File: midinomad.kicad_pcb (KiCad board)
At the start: 2 copper layers, 169.1 x 87.3 mm, 59 parts, among them J1 MIDI IN, J2 MIDI OUT, J3 Nomad 5pin, J4 Nomad 100, J7 DC IN, U1 6N138, U2 L7805, U3 74HC4053, U4 74HC4053

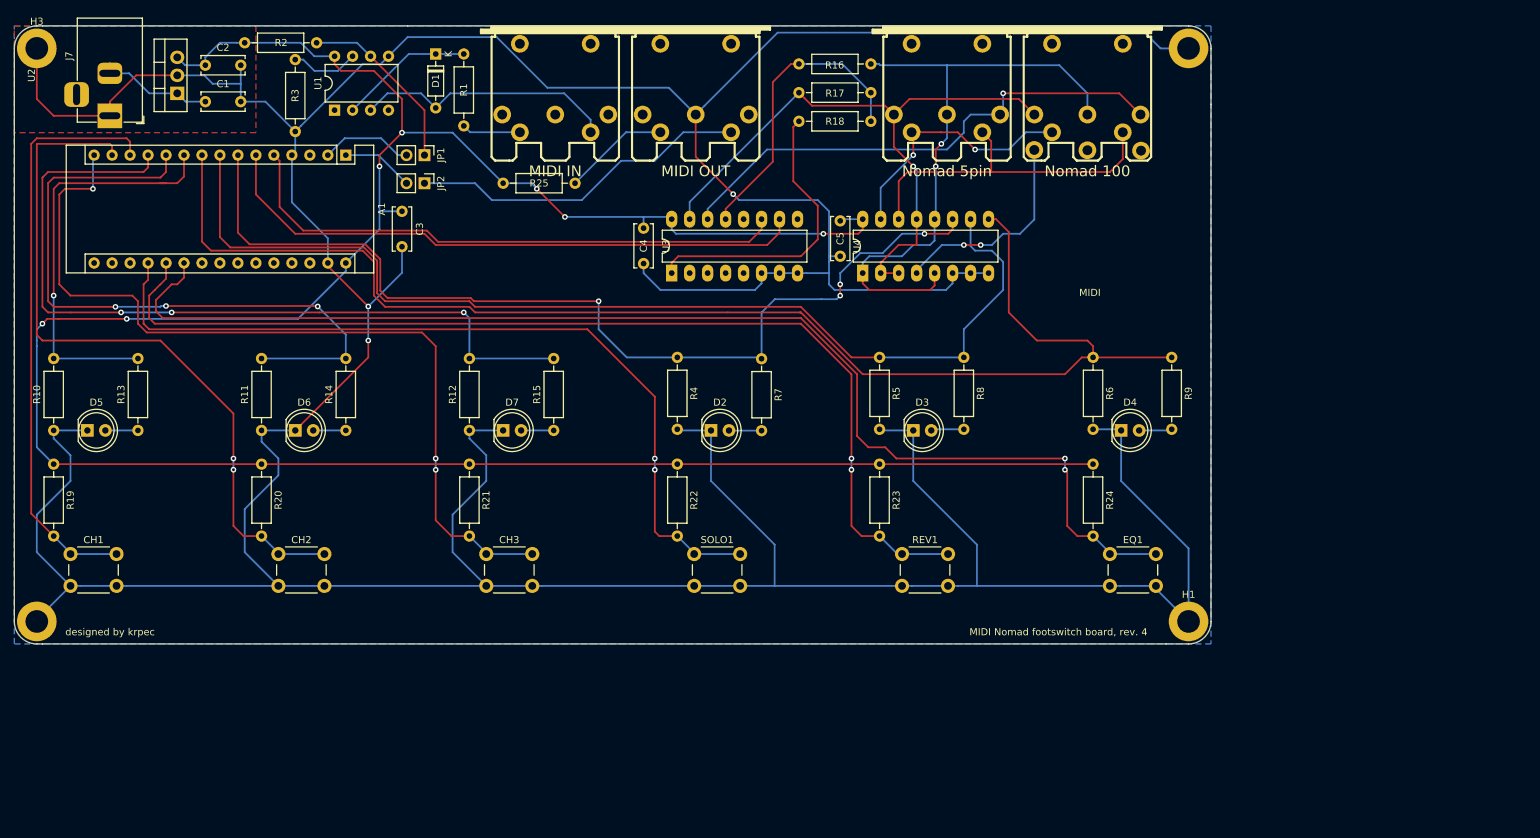
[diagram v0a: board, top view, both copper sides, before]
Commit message: Rev. 6 PCB & schematics
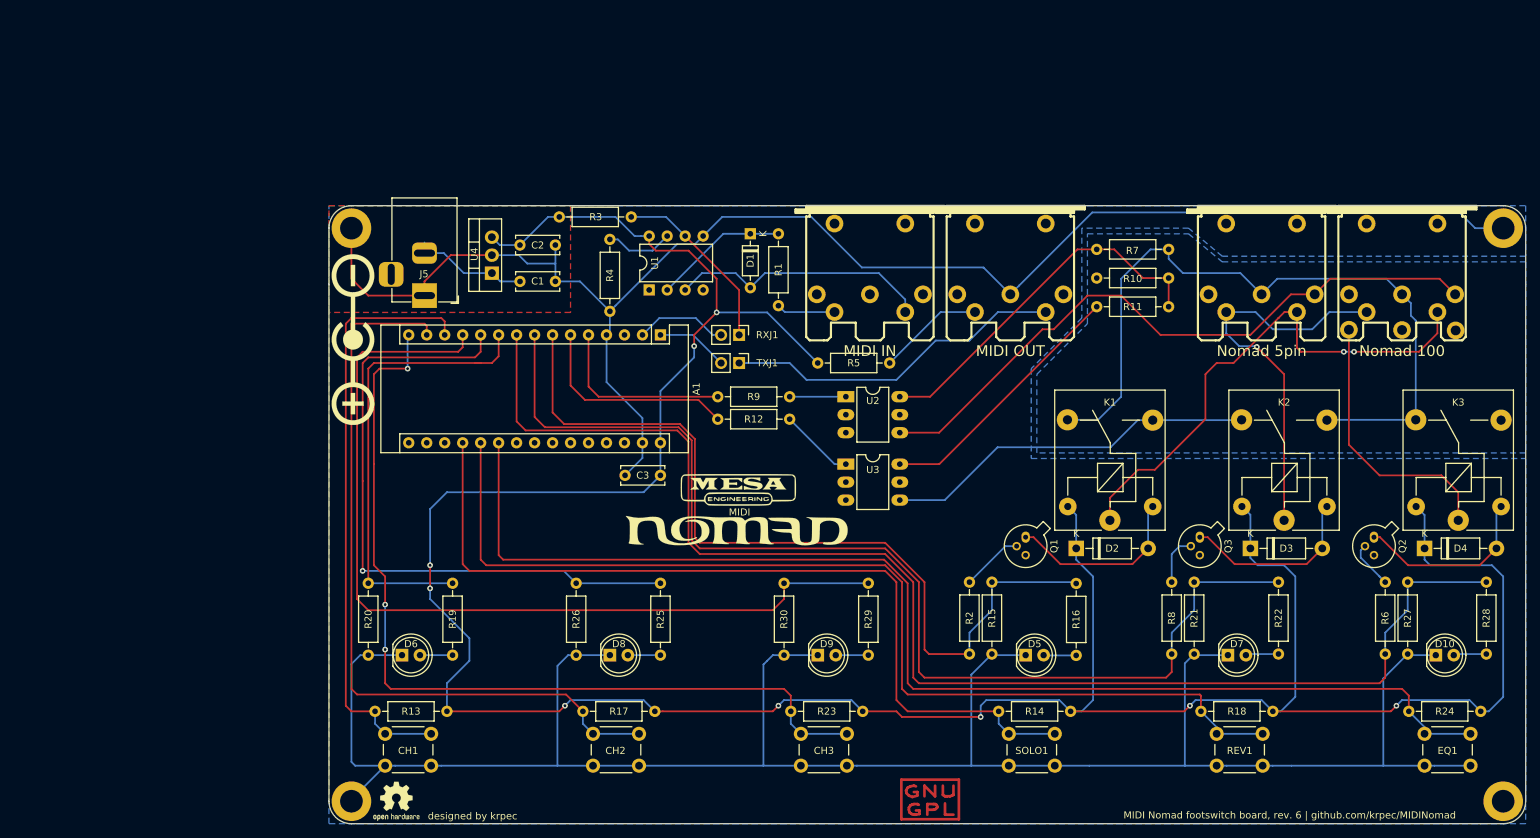
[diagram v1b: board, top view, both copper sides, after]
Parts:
- removed C4, C5: 0.1uF, Capacitor_THT:C_Disc_D6.0mm_W2.5mm_P5.00mm
- removed the U4 at (139.7, 57.1)
- added D10: LED, LED_THT:LED_D5.0mm, F.Cu at (220.7, 111.1)
- added D2: 1N4007, Diode_THT:D_DO-41_SOD81_P10.16mm_Horizontal, F.Cu at (169.9, 96.0)
- added D3: 1N4007, Diode_THT:D_DO-41_SOD81_P10.16mm_Horizontal, F.Cu at (194.5, 96.0)
- added G***: LOGO, midinomad-mux:board-logo, F.Cu at (122.2, 89.7)
- added K1: SANYOU_SRD_Form_C, Relay_THT:Relay_SPDT_SANYOU_SRD_Series_Form_C, F.Cu at (174.6, 92.1)
- added K2: SANYOU_SRD_Form_C, Relay_THT:Relay_SPDT_SANYOU_SRD_Series_Form_C, F.Cu at (199.2, 92.1)
- added K3: SANYOU_SRD_Form_C, Relay_THT:Relay_SPDT_SANYOU_SRD_Series_Form_C, F.Cu at (223.8, 92.1)
- added Q1: 2N2222, Package_TO_SOT_THT:TO-18-3, F.Cu at (162.7, 94.5)
- added Q2: 2N2222, Package_TO_SOT_THT:TO-18-3, F.Cu at (211.9, 94.5)
- added Q3: 2N2222, Package_TO_SOT_THT:TO-18-3, F.Cu at (187.3, 94.5)
- added R12: 220R, Resistor_THT:R_Axial_DIN0207_L6.3mm_D2.5mm_P10.16mm_Horizontal, F.Cu at (129.4, 77.8)
- added R2: 1k, Resistor_THT:R_Axial_DIN0207_L6.3mm_D2.5mm_P10.16mm_Horizontal, F.Cu at (154.8, 100.8)
- added R27: 10k, Resistor_THT:R_Axial_DIN0207_L6.3mm_D2.5mm_P10.16mm_Horizontal, F.Cu at (216.7, 100.8)
- added R28: 220R, Resistor_THT:R_Axial_DIN0207_L6.3mm_D2.5mm_P10.16mm_Horizontal, F.Cu at (227.8, 100.8)
- added R8: 1k, Resistor_THT:R_Axial_DIN0207_L6.3mm_D2.5mm_P10.16mm_Horizontal, F.Cu at (183.4, 100.8)
- added REF**: Symbol_GNU-GPL_CopperTop_Small, Symbol:Symbol_GNU-GPL_CopperTop_Small, F.Cu at (149.2, 131.8)
- added REF**: Polarity_Center_Negative_6mm_SilkScreen, Symbol:Polarity_Center_Negative_6mm_SilkScreen, F.Cu at (67.7, 66.5)
- added REF**: OSHW-Logo2_7.3x6mm_SilkScreen, Symbol:OSHW-Logo2_7.3x6mm_SilkScreen, F.Cu at (73.8, 131.8)
- added U2: MOC3041M, Package_DIP:DIP-6_W7.62mm_LongPads, F.Cu at (137.3, 74.6)
- D4: value LED -> 1N4007; footprint LED_THT:LED_D5.0mm -> Diode_THT:D_DO-41_SOD81_P10.16mm_Horizontal
- R6: value 10k -> 1k
- U3: value 74HC4053 -> MOC3041M; footprint Package_DIP:DIP-16_W7.62mm_LongPads -> Package_DIP:DIP-6_W7.62mm_LongPads
- moved R13 65.6 mm to (81.0, 119.1), turned to 180 degrees
- moved R14 65.6 mm to (169.1, 119.1), turned to 180 degrees
- moved R17 65.6 mm to (110.3, 119.1), turned to 180 degrees
- moved R18 65.6 mm to (197.6, 119.1), turned to 180 degrees
- moved R23 65.6 mm to (139.7, 119.1), turned to 180 degrees
- moved R24 65.0 mm to (227.0, 119.1), turned to 180 degrees
- moved R15 54.6 mm to (158.0, 100.8)
- moved R16 54.6 mm to (169.9, 101.0)
- moved D5 54.6 mm to (162.7, 111.1)
- moved D8 54.6 mm to (104.0, 111.1)
- moved R25 54.6 mm to (111.1, 111.1)
- moved R26 54.6 mm to (99.2, 111.1)
- moved R29 54.6 mm to (140.5, 111.1)
- moved R30 54.6 mm to (128.6, 111.1)
- moved D6 54.6 mm to (74.6, 111.1)
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- renumbered D2 to D5, D5 to D6, D3 to D7, D6 to D8, D7 to D9, J3 to J2, J4 to J3, J2 to J4, J7 to J5, R17 to R10, R18 to R11, R19 to R13, R22 to R14, R4 to R15, R7 to R16, R20 to R17, R23 to R18, R13 to R19, R10 to R20, R5 to R21, R8 to R22, R21 to R23, R14 to R25, R11 to R26, R15 to R29, R2 to R3, R12 to R30, R3 to R4, R25 to R5, R16 to R7, JP1 to RXJ1, JP2 to TXJ1, U2 to U4
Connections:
- D4 pad 1: GNDREF -> +5V
- R10 pad 2: Net-(R16-Pad1) -> Net-(R10-Pad2)
- R11 pad 1: Net-(R18-Pad1) -> Net-(R11-Pad1)
- R11 pad 2: Net-(R16-Pad1) -> Net-(R10-Pad2)
- R6 pad 1: Arduino_D6 -> Net-(Q2-Pad2)
- R6 pad 2: GNDREF -> Arduino_D6
- R7 pad 1: Net-(R16-Pad1) -> Net-(R10-Pad2)
- R9 pad 1: Arduino_D6 -> Net-(R9-Pad1)
- R9 pad 2: Net-(D4-Pad2) -> Arduino_D2
- U3 pad 1: Net-(R18-Pad1) -> Net-(R12-Pad1)
- U3 pad 2: Net-(U3-Pad2) -> GNDREF
- U3 pad 4: Net-(U3-Pad4) -> -3V
- U3 pad 6: GNDREF -> Net-(R11-Pad1)
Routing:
- net GNDREF: track 712.6 -> 520.5 mm, vias 3 -> 0
- net +5V: track 361.3 -> 417.4 mm, vias 7 -> 9
- net Arduino_D3: track 85.1 -> 29.9 mm
- net Arduino_D2: track 80.0 -> 26.2 mm
- net Net-(R10-Pad2): track 0.00 -> 52.3 mm
- net Net-(R16-Pad1): track 42.8 -> 0.00 mm
- net Net-(R18-Pad1): track 41.9 -> 0.00 mm
- net -3V: track 90.5 -> 53.0 mm, vias 1 -> 0
- net Net-(R11-Pad1): track 0.00 -> 37.0 mm
- net Net-(D2-Pad2): track 0.00 -> 26.0 mm
- net Net-(D3-Pad2): track 0.00 -> 26.0 mm
- net MESA_SWA_(SOLO): track 48.3 -> 73.4 mm, vias 0 -> 2
- net Net-(D4-Pad2): track 4.89 -> 26.1 mm
- net MESA_VCH: track 73.0 -> 94.1 mm, vias 1 -> 0
- net MESA_SWB_(REV): track 36.1 -> 55.9 mm, vias 2 -> 1
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- added copper zone on B.Cu, net -3V
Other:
- board text added: "MIDI Nomad footswitch board, rev. 6 | github.com/krpec/MIDINomad"
- board text removed: "MIDI Nomad footswitch board, rev. 4"
